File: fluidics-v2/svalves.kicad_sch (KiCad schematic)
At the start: 0 parts

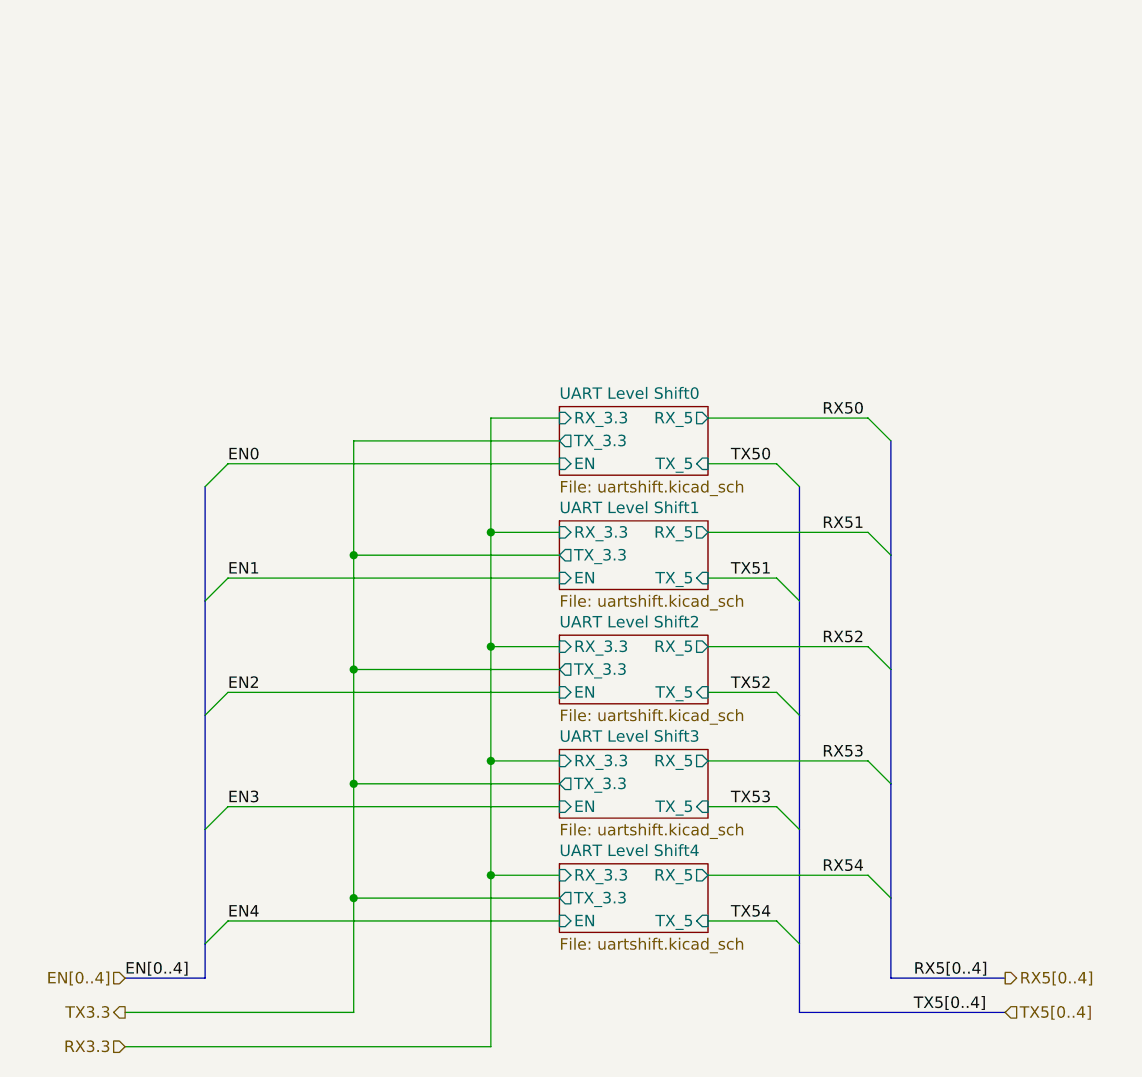
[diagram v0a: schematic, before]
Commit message: new version
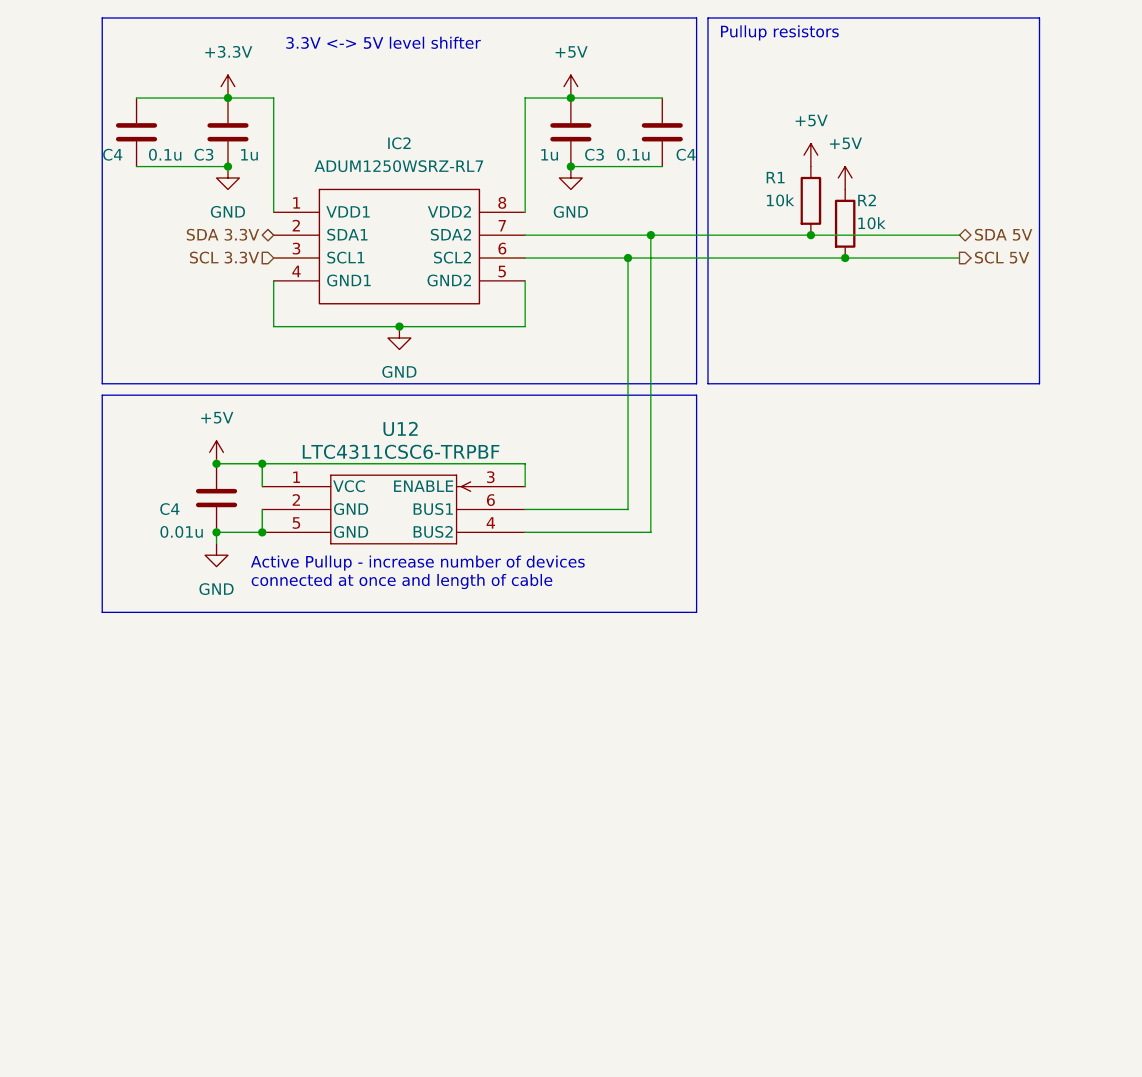
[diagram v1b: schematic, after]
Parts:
- added C3 (x2): 1u, Capacitor_SMD:C_0603_1608Metric, symbol Device:C
- added C4: 0.01u, Capacitor_SMD:C_0603_1608Metric, symbol Device:C
- added C4 (x2): 0.1u, Capacitor_SMD:C_0603_1608Metric, symbol Device:C
- added IC2: ADUM1250WSRZ-RL7, analog_devices:SOIC127P600X175-8N, symbol analog_devices:ADUM1250WSRZ-RL7
- added R1, R2: 10k, Resistor_SMD:R_0402_1005Metric, symbol Device:R
- added U12: LTC4311CSC6-TRPBF, SOT-6_SC_LIT, symbol LTC4311CSC6#TRPBF:LTC4311CSC6-TRPBF
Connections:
- new net +3.3V: C3.1, C4.1, IC2.1 (VDD1)
- new net +5V: C3.1, C4.1, C4.1, IC2.8 (VDD2), R1.1, R2.1, U12.1 (VCC), U12.3 (ENABLE)
- new net GND: C3.2, C3.2, C4.2, C4.2, C4.2, IC2.4 (GND1), IC2.5 (GND2), U12.2 (GND), U12.5 (GND)
- new net SCL 3.3V: IC2.3 (SCL1)
- new net SCL 5V: IC2.6 (SCL2), R2.2, U12.6 (BUS1)
- new net SDA 3.3V: IC2.2 (SDA1)
- new net SDA 5V: IC2.7 (SDA2), R1.2, U12.4 (BUS2)
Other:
- removed sheet UART Level Shift0
- removed sheet UART Level Shift1
- removed sheet UART Level Shift2
- removed sheet UART Level Shift3
- removed sheet UART Level Shift4
- note added: "3.3V <-> 5V level shifter"
- note added: "Active Pullup - increase number of devices connected at once and length of cable"
- note added: "Pullup resistors"
